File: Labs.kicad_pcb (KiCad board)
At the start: 2 copper layers, 46.5 x 34.8 mm, 29 parts, among them J1 Conn_02x05_Counter_Clockwise, SW1BOOT1 SW_Push, SW2NRST1 SW_Push, U1 STM32F407VGTx, Y1 Crystal

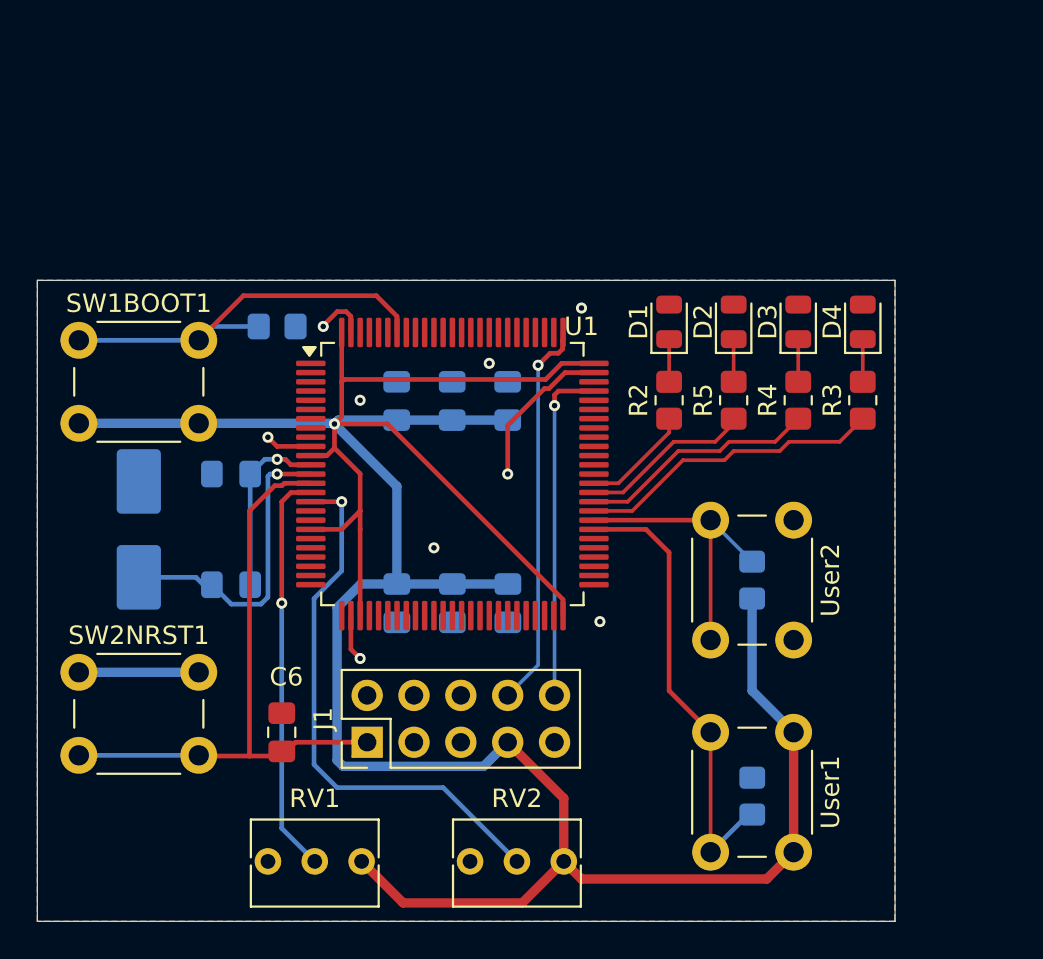
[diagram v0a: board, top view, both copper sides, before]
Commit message: feat: add tracing
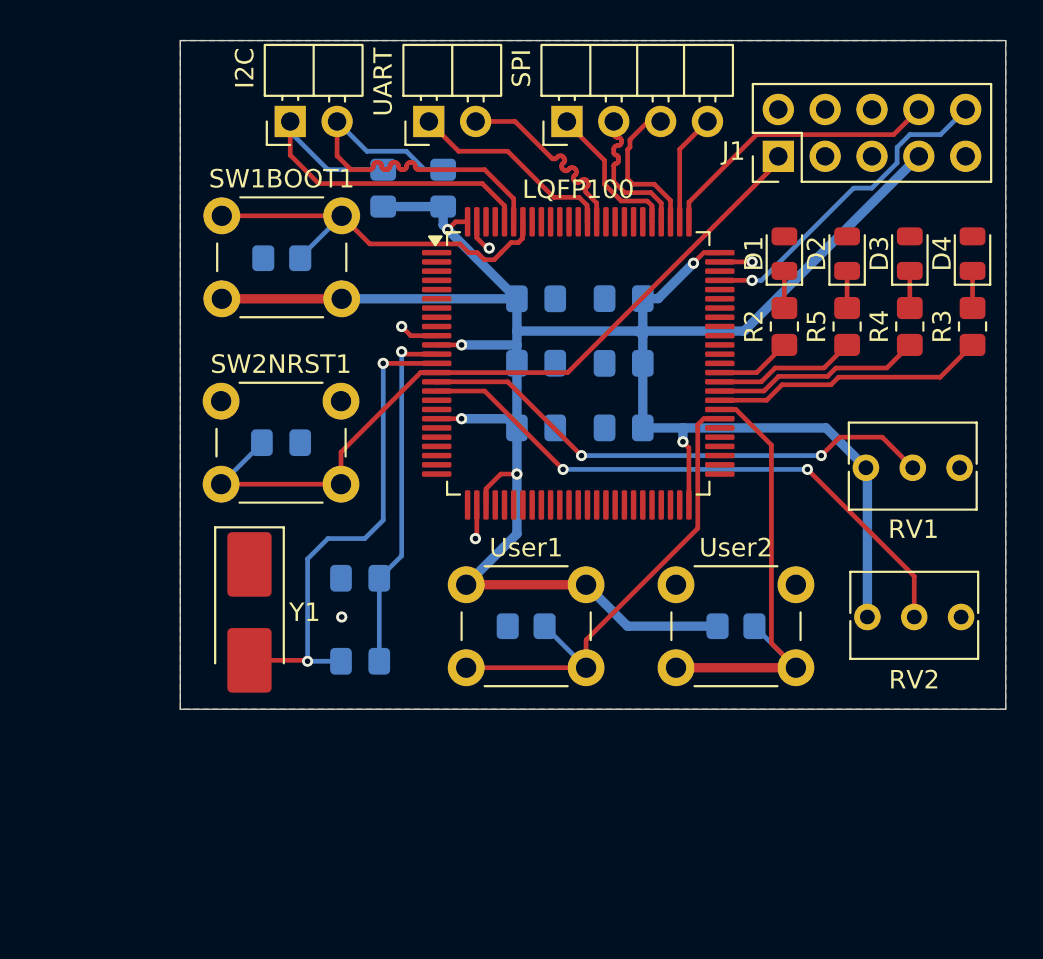
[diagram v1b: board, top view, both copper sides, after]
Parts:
- removed U1: STM32F407VGTx, Package_QFP:LQFP-100_14x14mm_P0.5mm
- added I2C: Conn_01x02_Pin, Connector_PinHeader_2.54mm:PinHeader_1x02_P2.54mm_Horizontal, F.Cu at (131.2, 78.9)
- added LQFP100: STM32F407VGTx, Package_QFP:LQFP-100_14x14mm_P0.5mm, F.Cu at (146.8, 92.0)
- added R8: R 2.2 kOhm, Resistor_SMD:R_0805_2012Metric_Pad1.20x1.40mm_HandSolder, B.Cu at (139.5, 82.5)
- added R9: R 2.2 kOhm, Resistor_SMD:R_0805_2012Metric_Pad1.20x1.40mm_HandSolder, B.Cu at (136.2, 82.5)
- added SPI: Conn_01x04_Pin, Connector_PinHeader_2.54mm:PinHeader_1x04_P2.54mm_Horizontal, F.Cu at (146.2, 78.9)
- added UART: Conn_01x02_Pin, Connector_PinHeader_2.54mm:PinHeader_1x02_P2.54mm_Horizontal, F.Cu at (138.7, 78.9)
- C6: moved to B.Cu
- J1: value Conn_02x05_Counter_Clockwise -> PROG_port
- Y1: moved to F.Cu
- moved J1 38.8 mm to (157.7, 80.8)
- moved RV1 34.7 mm to (162.4, 97.7), turned to 180 degrees
- moved RV2 21.1 mm to (162.5, 105.8), turned to 180 degrees
- moved User1 19.5 mm to (140.8, 104.0), turned to 0 degrees
- moved C1 18.1 mm to (144.5, 88.5), turned to 180 degrees
- moved SW2NRST1 16.6 mm to (127.5, 94.0)
- moved C6 15.7 mm to (130.7, 96.3), turned to 180 degrees
- moved R6 15.3 mm to (144.0, 106.2), turned to 180 degrees
- moved C2 13.8 mm to (144.5, 92.0), turned to 180 degrees
- moved C7 13.5 mm to (149.3, 88.5), turned to 0 degrees
- moved SW1BOOT1 10.3 mm to (127.5, 84.0)
- moved C3 9.62 mm to (144.5, 95.5), turned to 180 degrees
- moved C8 9.52 mm to (149.3, 92.0), turned to 0 degrees
- moved C5 9.00 mm to (135.0, 103.7)
- moved C4 8.14 mm to (135.0, 108.2)
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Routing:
- net +3.3V: track 162.2 -> 133.6 mm, vias 1 -> 6
- net /I2C_SDA: track 0.00 -> 21.9 mm
- net /I2C_SCL: track 0.00 -> 21.8 mm
- net GND: track 22.9 -> 7.49 mm, vias 9 -> 5
- net /UART_RX: track 0.00 -> 11.4 mm
- net /UART_TX: track 0.00 -> 11.3 mm
- net /UButton_2: track 16.0 -> 25.9 mm
- net /EXTAL: track 17.3 -> 26.9 mm, vias 1 -> 2
- net /XTAL: track 10.1 -> 19.2 mm
- net /SPI_SCK: track 0.00 -> 8.25 mm
- net /SPI_MOSI: track 0.00 -> 8.20 mm
- net /SPI_MISO: track 0.00 -> 8.15 mm
- net /NRST: track 34.3 -> 41.9 mm
- net /ADC_1: track 22.0 -> 28.6 mm, vias 1 -> 2
- net /SPI_NSS: track 0.00 -> 6.06 mm
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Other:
- board size 46.5 x 34.8 mm -> 44.8 x 36.2 mm
